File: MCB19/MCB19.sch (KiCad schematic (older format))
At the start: 1 part

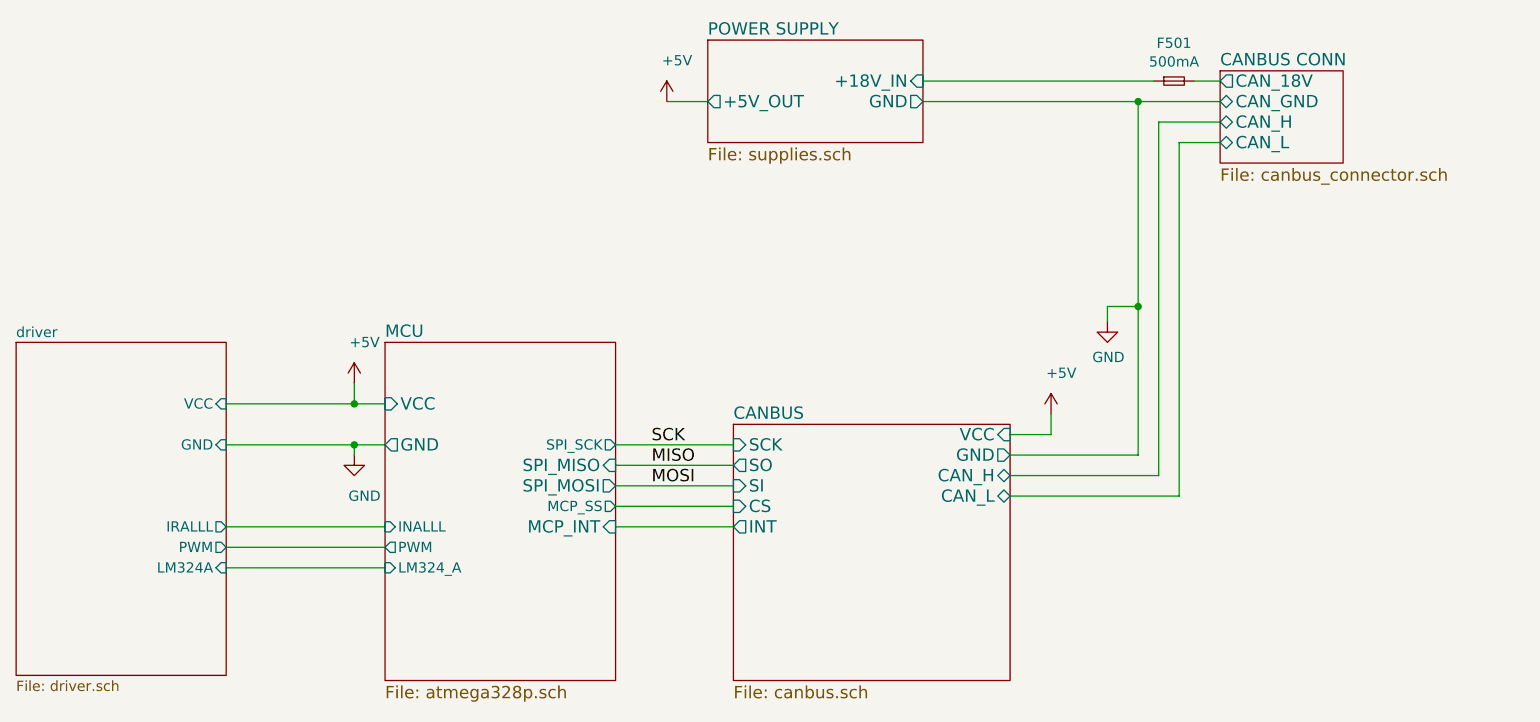
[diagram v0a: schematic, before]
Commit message: Final!!!
Pronto para fabricar
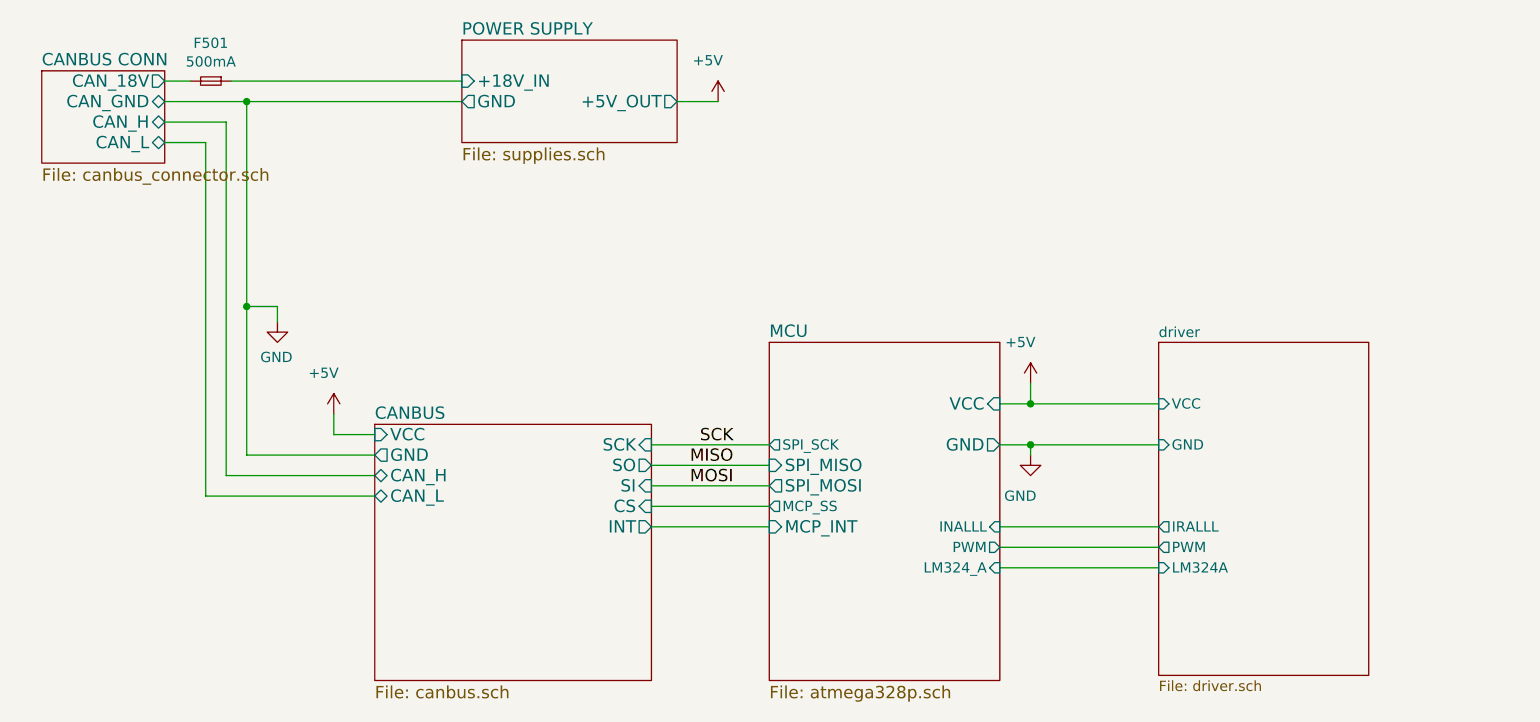
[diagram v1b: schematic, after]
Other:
- moved on the sheet: F501
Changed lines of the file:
@@
 $EndDescr
 $Sheet
-S 7300 2750 1350 1250
+S 5550 2750 1350 1250
 U 5AABFC1B
 F0 "CANBUS" 60
 F1 "canbus.sch" 60
-F2 "SI" I L 7300 3050 60
-F3 "SO" O L 7300 2950 60
-F4 "CS" I L 7300 3150 60
-F5 "SCK" I L 7300 2850 60
-F6 "INT" O L 7300 3250 60
-F7 "GND" O R 8650 2900 60
-F8 "VCC" I R 8650 2800 60
-F9 "CAN_H" B R 8650 3000 60
-F10 "CAN_L" B R 8650 3100 60
-$EndSheet
-$Sheet
-S 7175 875  1050 500
+F2 "SI" I R 6900 3050 60
+F3 "SO" O R 6900 2950 60
+F4 "CS" I R 6900 3150 60
+F5 "SCK" I R 6900 2850 60
+F6 "INT" O R 6900 3250 60
+F7 "GND" O L 5550 2900 60
+F8 "VCC" I L 5550 2800 60
+F9 "CAN_H" B L 5550 3000 60
+F10 "CAN_L" B L 5550 3100 60
+$EndSheet
+$Sheet
+S 5975 875  1050 500
 U 5AACFFEF
 F0 "POWER SUPPLY" 60
 F1 "supplies.sch" 60
-F2 "GND" O R 8225 1175 60
-F3 "+5V_OUT" O L 7175 1175 60
-F4 "+18V_IN" I R 8225 1075 60
-$EndSheet
-$Sheet
-S 9675 1025 600  450
+F2 "GND" O L 5975 1175 60
+F3 "+5V_OUT" O R 7025 1175 60
+F4 "+18V_IN" I L 5975 1075 60
+$EndSheet
+$Sheet
+S 3925 1025 600  450
 U 5AAD16DD
 F0 "CANBUS CONN" 60
 F1 "canbus_connector.sch" 60
-F2 "CAN_H" B L 9675 1275 60
-F3 "CAN_L" B L 9675 1375 60
-F4 "CAN_18V" O L 9675 1075 60
-F5 "CAN_GND" B L 9675 1175 60
-$EndSheet
-Text Label 6900 3050 0    60   ~ 0
+F2 "CAN_H" B R 4525 1275 60
+F3 "CAN_L" B R 4525 1375 60
+F4 "CAN_18V" O R 4525 1075 60
+F5 "CAN_GND" B R 4525 1175 60
+$EndSheet
+Text Label 7300 3050 2    60   ~ 0
 MOSI
-Text Label 6900 2950 0    60   ~ 0
+Text Label 7300 2950 2    60   ~ 0
 MISO
-Text Label 6900 2850 0    60   ~ 0
+Text Label 7300 2850 2    60   ~ 0
 SCK
 Wire Wire Line
-	9675 1275 9375 1275
-Wire Wire Line
-	8650 3100 9475 3100
-Wire Wire Line
-	9475 1375 9675 1375
-Connection ~ 9275 1175
-Wire Wire Line
-	7175 1175 6975 1175
-Wire Wire Line
-	8850 2800 8650 2800
-Wire Wire Line
-	9275 1175 9675 1175
+	4525 1275 4825 1275
+Wire Wire Line
+	5550 3100 4725 3100
+Wire Wire Line
+	4725 1375 4525 1375
+Connection ~ 4925 1175
+Wire Wire Line
+	7025 1175 7225 1175
+Wire Wire Line
+	5350 2800 5550 2800
+Wire Wire Line
+	4925 1175 4525 1175
 $Comp
 L power:+5V #PWR0105
 U 1 1 5BE8FCAE
-P 8850 2700
-F 0 "#PWR0105" H 8850 2550 50  0001 C CNN
-F 1 "+5V" H 8900 2900 50  0000 C CNN
-F 2 "" H 8850 2700 50  0001 C CNN
-F 3 "" H 8850 2700 50  0001 C CNN
-	1    8850 2700
-	1    0    0    -1
+P 5350 2700
+F 0 "#PWR0105" H 5350 2550 50  0001 C CNN
+F 1 "+5V" H 5400 2900 50  0000 C CNN
+F 2 "" H 5350 2700 50  0001 C CNN
+F 3 "" H 5350 2700 50  0001 C CNN
+	1    5350 2700
+	-1   0    0    -1
 $EndComp
 $Comp
 L power:+5V #PWR0104
 U 1 1 5C9032F1
-P 5450 2550
-F 0 "#PWR0104" H 5450 2400 50  0001 C CNN
-F 1 "+5V" H 5500 2750 50  0000 C CNN
-F 2 "" H 5450 2550 50  0001 C CNN
-F 3 "" H 5450 2550 50  0001 C CNN
-	1    5450 2550
-	1    0    0    -1
-$EndComp
-Wire Wire Line
-	5450 2550 5450 2650
-Wire Wire Line
-	5450 2650 5600 2650
+P 8750 2550
+F 0 "#PWR0104" H 8750 2400 50  0001 C CNN
+F 1 "+5V" H 8800 2750 50  0000 C CNN
+F 2 "" H 8750 2550 50  0001 C CNN
+F 3 "" H 8750 2550 50  0001 C CNN
+	1    8750 2550
+	-1   0    0    -1
+$EndComp
+Wire Wire Line
+	8750 2550 8750 2650
+Wire Wire Line
+	8750 2650 8600 2650
 $Comp
 L power:GND #PWR0106
 U 1 1 5C9038CC
-P 5450 2900
-F 0 "#PWR0106" H 5450 2650 50  0001 C CNN
-F 1 "GND" H 5500 2700 50  0000 C CNN
-F 2 "" H 5450 2900 50  0001 C CNN
-F 3 "" H 5450 2900 50  0001 C CNN
-	1    5450 2900
-	1    0    0    -1
-$EndComp
-Wire Wire Line
-	5450 2900 5450 2850
-Wire Wire Line
-	5450 2850 5600 2850
+P 8750 2900
+F 0 "#PWR0106" H 8750 2650 50  0001 C CNN
+F 1 "GND" H 8800 2700 50  0000 C CNN
+F 2 "" H 8750 2900 50  0001 C CNN
+F 3 "" H 8750 2900 50  0001 C CNN
+	1    8750 2900
+	-1   0    0    -1
+$EndComp
+Wire Wire Line
+	8750 2900 8750 2850
+Wire Wire Line
+	8750 2850 8600 2850
 $Comp
 L power:+5V #PWR0102
 U 1 1 5CDDDD31
-P 6975 1175
-F 0 "#PWR0102" H 6975 1025 50  0001 C CNN
-F 1 "+5V" H 7025 1375 50  0000 C CNN
-F 2 "" H 6975 1175 50  0001 C CNN
-F 3 "" H 6975 1175 50  0001 C CNN
-	1    6975 1175
-	1    0    0    -1
+P 7225 1175
+F 0 "#PWR0102" H 7225 1025 50  0001 C CNN
+F 1 "+5V" H 7275 1375 50  0000 C CNN
+F 2 "" H 7225 1175 50  0001 C CNN
+F 3 "" H 7225 1175 50  0001 C CNN
+	1    7225 1175
+	-1   0    0    -1
 $EndComp
 $Comp
 L power:GND #PWR0103
 U 1 1 5CDE058E
-P 9125 2250
-F 0 "#PWR0103" H 9125 2000 50  0001 C CNN
-F 1 "GND" H 9130 2077 50  0000 C CNN
-F 2 "" H 9125 2250 50  0001 C CNN
-F 3 "" H 9125 2250 50  0001 C CNN
-	1    9125 2250
-	1    0    0    -1
-$EndComp
-Wire Wire Line
-	9125 2250 9125 2175
-Wire Wire Line
-	9125 2175 9275 2175
-Wire Wire Line
-	8850 2700 8850 2800
-Wire Wire Line
-	9275 2175 9275 2900
-Connection ~ 9275 2175
-Wire Wire Line
-	8650 2900 9275 2900
-Wire Wire Line
-	9375 1275 9375 3000
-Wire Wire Line
-	9375 3000 8650 3000
-Wire Wire Line
-	9475 1375 9475 3100
-Wire Wire Line
-	8225 1175 9275 1175
+P 5075 2250
+F 0 "#PWR0103" H 5075 2000 50  0001 C CNN
+F 1 "GND" H 5080 2077 50  0000 C CNN
+F 2 "" H 5075 2250 50  0001 C CNN
+F 3 "" H 5075 2250 50  0001 C CNN
+	1    5075 2250
+	-1   0    0    -1
+$EndComp
+Wire Wire Line
+	5075 2250 5075 2175
+Wire Wire Line
+	5075 2175 4925 2175
+Wire Wire Line
+	5350 2700 5350 2800
+Wire Wire Line
+	4925 2175 4925 2900
+Connection ~ 4925 2175
+Wire Wire Line
+	5550 2900 4925 2900
+Wire Wire Line
+	4825 1275 4825 3000
+Wire Wire Line
+	4825 3000 5550 3000
+Wire Wire Line
+	4725 1375 4725 3100
+Wire Wire Line
+	5975 1175 4925 1175
 $Comp
 L Device:Fuse_Small F501
 U 1 1 5CDF621D
-P 9450 1075
-F 0 "F501" H 9450 1260 50  0000 C CNN
-F 1 "500mA" H 9450 1169 50  0000 C CNN
-F 2 "Fuse:Fuse_1206_3216Metric_Pad1.42x1.75mm_HandSolder" H 9450 1075 50  0001 C CNN
-F 3 "~" H 9450 1075 50  0001 C CNN
-	1    9450 1075
-	1    0    0    -1
-$EndComp
-Wire Wire Line
-	9550 1075 9675 1075
-Wire Wire Line
-	6725 2850 7300 2850
-Wire Wire Line
-	6725 2950 7300 2950
-Wire Wire Line
-	6725 3050 7300 3050
-Wire Wire Line
-	6725 3150 7300 3150
-Wire Wire Line
-	6725 3250 7300 3250
-$Sheet
-S 5600 2350 1125 1650
+P 4750 1075
+F 0 "F501" H 4750 1260 50  0000 C CNN
+F 1 "500mA" H 4750 1169 50  0000 C CNN
+F 2 "Fuse:Fuse_1206_3216Metric_Pad1.42x1.75mm_HandSolder" H 4750 1075 50  0001 C CNN
+F 3 "~" H 4750 1075 50  0001 C CNN
+	1    4750 1075
+	-1   0    0    -1
+$EndComp
+Wire Wire Line
+	4650 1075 4525 1075
+Wire Wire Line
+	7475 2850 6900 2850
+Wire Wire Line
+	7475 2950 6900 2950
+Wire Wire Line
+	7475 3050 6900 3050
+Wire Wire Line
+	7475 3150 6900 3150
+Wire Wire Line
+	7475 3250 6900 3250
+$Sheet
+S 7475 2350 1125 1650
 U 5AACA401
 F0 "MCU" 60
 F1 "atmega328p.sch" 60
-F2 "SPI_MISO" I R 6725 2950 60
-F3 "SPI_MOSI" O R 6725 3050 60
-F4 "MCP_INT" I R 6725 3250 60
-F5 "VCC" I L 5600 2650 60
-F6 "GND" O L 5600 2850 60
-F7 "SPI_SCK" O R 6725 2850 50
-F8 "MCP_SS" O R 6725 3150 50
-F9 "INALLL" I L 5600 3250 50
-F10 "PWM" O L 5600 3350 50
-F11 "LM324_A" I L 5600 3450 50
-$EndSheet
-$Sheet
-S 3800 2350 1025 1625
+F2 "SPI_MISO" I L 7475 2950 60
+F3 "SPI_MOSI" O L 7475 3050 60
+F4 "MCP_INT" I L 7475 3250 60
+F5 "VCC" I R 8600 2650 60
+F6 "GND" O R 8600 2850 60
+F7 "SPI_SCK" O L 7475 2850 50
+F8 "MCP_SS" O L 7475 3150 50
+F9 "INALLL" I R 8600 3250 50
+F10 "PWM" O R 8600 3350 50
+F11 "LM324_A" I R 8600 3450 50
+$EndSheet
+$Sheet
+S 9375 2350 1025 1625
 U 5D414D87
 F0 "driver" 50
 F1 "driver.sch" 50
-F2 "VCC" I R 4825 2650 50
-F3 "GND" I R 4825 2850 50
-F4 "IRALLL" O R 4825 3250 50
-F5 "PWM" O R 4825 3350 50
-F6 "LM324A" I R 4825 3450 50
-$EndSheet
-Wire Wire Line
-	9275 1175 9275 2175
-Wire Wire Line
-	8225 1075 9350 1075
-Wire Wire Line
-	4825 3250 5600 3250
-Wire Wire Line
-	5600 3350 4825 3350
-Wire Wire Line
-	5600 3450 4825 3450
-Wire Wire Line
-	5450 2850 4825 2850
-Connection ~ 5450 2850
-Wire Wire Line
-	4825 2650 5450 2650
-Connection ~ 5450 2650
+F2 "VCC" I L 9375 2650 50
+F3 "GND" I L 9375 2850 50
+F4 "IRALLL" O L 9375 3250 50
+F5 "PWM" O L 9375 3350 50
+F6 "LM324A" I L 9375 3450 50
+$EndSheet
+Wire Wire Line
+	4925 1175 4925 2175
+Wire Wire Line
+	5975 1075 4850 1075
+Wire Wire Line
+	9375 3250 8600 3250
+Wire Wire Line
+	8600 3350 9375 3350
+Wire Wire Line
+	8600 3450 9375 3450
+Wire Wire Line
+	8750 2850 9375 2850
+Connection ~ 8750 2850
+Wire Wire Line
+	9375 2650 8750 2650
+Connection ~ 8750 2650
 $EndSCHEMATC

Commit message: New version
Detalhes
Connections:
- net labels added: +15V
- wire segments 32 -> 39
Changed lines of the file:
@@
 $Descr A4 11693 8268
 encoding utf-8
-Sheet 1 6
+Sheet 1 7
 Title ""
 Date ""
@@
 Wire Wire Line
 	4725 1375 4525 1375
-Connection ~ 4925 1175
 Wire Wire Line
 	7025 1175 7225 1175
@@
 F5 "PWM" O L 9375 3350 50
 F6 "LM324A" I L 9375 3450 50
-$EndSheet
-Wire Wire Line
-	4925 1175 4925 2175
-Wire Wire Line
-	5975 1075 4850 1075
+F7 "+15V" I L 9375 2450 50
+$EndSheet
+Wire Wire Line
+	4925 1175 4925 1850
+Wire Wire Line
+	5975 1075 5025 1075
 Wire Wire Line
 	9375 3250 8600 3250
@@
 	9375 2650 8750 2650
 Connection ~ 8750 2650
+Connection ~ 4925 1175
+Wire Wire Line
+	5975 1850 4925 1850
+Connection ~ 4925 1850
+Wire Wire Line
+	4925 1850 4925 2175
+Wire Wire Line
+	5975 1750 5025 1750
+Wire Wire Line
+	5025 1750 5025 1075
+Connection ~ 5025 1075
+Wire Wire Line
+	5025 1075 4850 1075
+$Comp
+L power:+15V #PWR0109
+U 1 1 5D9C5743
+P 7225 1850
+F 0 "#PWR0109" H 7225 1700 50  0001 C CNN
+F 1 "+15V" H 7240 2023 50  0000 C CNN
+F 2 "" H 7225 1850 50  0001 C CNN
+F 3 "" H 7225 1850 50  0001 C CNN
+	1    7225 1850
+	1    0    0    -1
+$EndComp
+Wire Wire Line
+	7025 1850 7225 1850
+$Comp
+L power:+15V #PWR0112
+U 1 1 5DA06051
+P 9175 2450
+F 0 "#PWR0112" H 9175 2300 50  0001 C CNN
+F 1 "+15V" H 9190 2623 50  0000 C CNN
+F 2 "" H 9175 2450 50  0001 C CNN
+F 3 "" H 9175 2450 50  0001 C CNN
+	1    9175 2450
+	1    0    0    -1
+$EndComp
+Wire Wire Line
+	9175 2450 9375 2450
+$Sheet
+S 5975 1525 1050 500
+U 5DA09AB7
+F0 "supplies15" 50
+F1 "+15V.sch" 50
+F2 "GND" O L 5975 1850 50
+F3 "+15V_OUT" I R 7025 1850 50
+F4 "+18V_IN" I L 5975 1750 50
+$EndSheet
 $EndSCHEMATC
